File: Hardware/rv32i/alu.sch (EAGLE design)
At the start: 81 parts, among them IC1 SN74HCS86DR, IC10 SN74HCS86DR, IC11 SN74HCS86DR, IC12 SN74HCS86DR, IC13 SN74HCS86DR, IC14 SN74HCS86DR, IC15 SN74HCS86DR, IC16 SN74HCS86DR, IC17 SN74HCS86DR, IC18 SN74HCS86DR, IC19 SN74HCS86DR, IC2 SN74HCS86DR, IC20 SN74HCS86DR, IC21 SN74HCS86DR, IC22 SN74HCS86DR, IC23 SN74HCS86DR, IC24 SN74HCS86DR, IC25 SN74ACT08D, IC26 SN74ACT08D, IC27 SN74ACT08D, IC28 SN74ACT08D, IC29 SN74ACT08D, IC3 SN74HCS86DR, IC30 SN74ACT08D, IC31 SN74ACT08D, IC32 SN74ACT08D, IC33 SN74ACT08D, IC34 SN74ACT08D, IC35 SN74ACT08D, IC36 SN74ACT08D, IC37 SN74ACT08D, IC38 SN74ACT08D, IC39 SN74ACT08D, IC4 SN74HCS86DR, IC40 SN74ACT08D, IC41 SN74HCS32DR, IC42 SN74HCS32DR, IC43 SN74HCS32DR, IC44 SN74HCS32DR, IC45 SN74HCS32DR, IC46 SN74HCS32DR, IC47 SN74HCS32DR, IC48 SN74HCS32DR, IC5 SN74HCS86DR, IC6 SN74HCS86DR, IC7 SN74HCS86DR, IC8 SN74HCS86DR, IC9 SN74HCS86DR

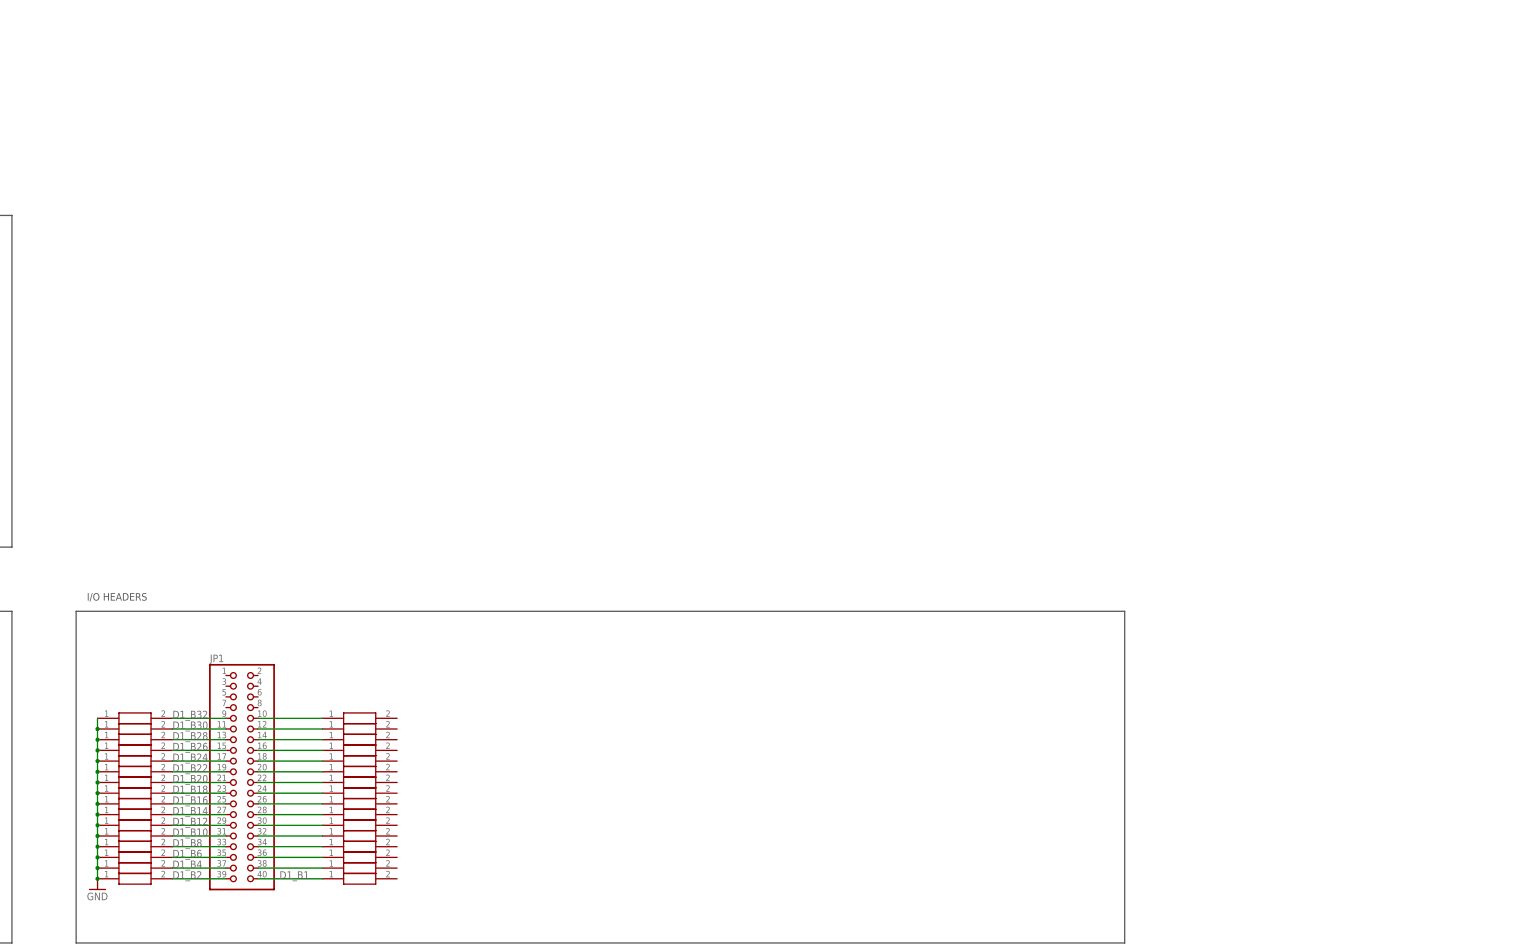
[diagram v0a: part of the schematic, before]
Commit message: ALU Headers & Timing Gates
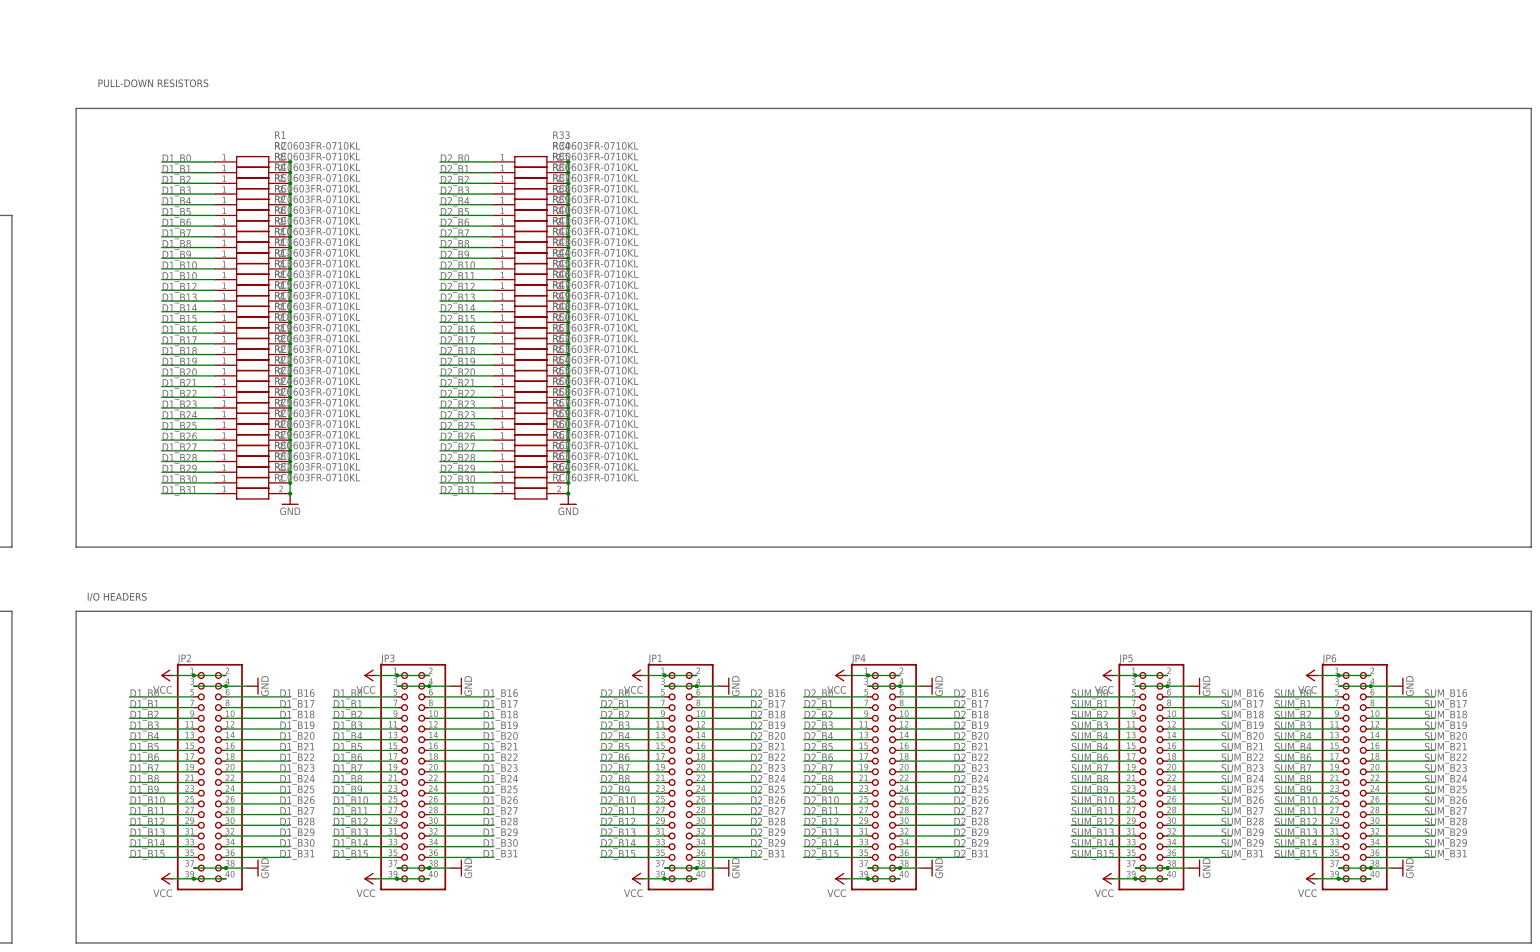
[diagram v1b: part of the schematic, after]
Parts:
- added JP2, JP3, JP4, JP5, JP6: (no value), pinhead:PINHD-2X20
- added R33, R34, R35, R36, R37, R38, R39, R40, R41, R42, R43, R44, R45, R46, R47, R48, R49, R50, R51, R52, R53, R54, R55, R56, R57, R58, R59, R60, R61, R62, R63, R64: RC0603FR-0710KL, RC0603FR-0710KL:RC0603FR-0710KL
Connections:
- removed net N$10: JP1.22, R26.1
- removed net N$11: JP1.24, R25.1
- removed net N$12: JP1.26, R17.1
- removed net N$13: JP1.28, R18.1
- removed net N$14: JP1.30, R19.1
- removed net N$16: JP1.32, R20.1
- removed net N$17: JP1.34, R22.1
- removed net N$18: JP1.36, R21.1
- removed net N$19: JP1.38, R23.1
- removed net N$2: JP1.10, R31.1
- removed net N$4: JP1.12, R32.1
- removed net N$5: JP1.14, R30.1
- removed net N$6: JP1.16, R29.1
- removed net N$7: JP1.18, R28.1
- removed net N$9: JP1.20, R27.1
- new net D1_B0: JP2.5, JP3.5, R1.1
- new net D2_B0: JP1.5, JP4.5, R33.1
- new net SUM_B0: JP5.5, JP6.5
- new net VCC: JP1.1, JP1.2, JP1.39, JP1.40, JP2.1, JP2.2, JP2.39, JP2.40, JP3.1, JP3.2, JP3.39, JP3.40, JP4.1, JP4.2, JP4.39, JP4.40, JP5.1, JP5.2, JP5.39, JP5.40, JP6.1, JP6.2, JP6.39, JP6.40
- net D1_B1: now also JP2.7, JP3.7, R2.1; no longer JP1.40, R24.1
- net D1_B10: now also JP2.25, JP3.25, R11.1, R12.1; no longer JP1.31, R4.2
- net D1_B11: now also JP2.27, JP3.27
- net D1_B12: now also JP2.29, JP3.29, R13.1; no longer JP1.29, R3.2
- net D1_B13: now also JP2.31, JP3.31, R14.1
- net D1_B14: now also JP2.33, JP3.33, R15.1; no longer JP1.27, R2.2
- net D1_B15: now also JP2.35, JP3.35, R17.1
- net D1_B16: now also JP2.6, JP3.6, R16.1; no longer JP1.25, R1.2
- net D1_B17: now also JP2.8, JP3.8, R18.1
- net D1_B18: now also JP2.10, JP3.10, R19.1; no longer JP1.23, R9.2
- net D1_B19: now also JP2.12, JP3.12, R20.1
- net D1_B2: now also JP2.9, JP3.9, R3.1; no longer JP1.39, R8.2
- net D1_B20: now also JP2.14, JP3.14, R21.1; no longer JP1.21, R10.2
- net D1_B21: now also JP2.16, JP3.16, R22.1
- net D1_B22: now also JP2.18, JP3.18, R23.1; no longer JP1.19, R11.2
- net D1_B23: now also JP2.20, JP3.20, R24.1
- net D1_B24: now also JP2.22, JP3.22, R26.1; no longer JP1.17, R12.2
- net D1_B25: now also JP2.24, JP3.24, R25.1
- net D1_B26: now also JP2.26, JP3.26, R27.1; no longer JP1.15, R13.2
- net D1_B27: now also JP2.28, JP3.28, R28.1
- net D1_B28: now also JP2.30, JP3.30, R29.1; no longer JP1.13, R14.2
- net D1_B29: now also JP2.32, JP3.32, R30.1
- net D1_B3: now also JP2.11, JP3.11, R4.1
- net D1_B30: now also JP2.34, JP3.34, R31.1; no longer JP1.11, R16.2
- net D1_B31: now also JP2.36, JP3.36, R32.1
- net D1_B32: no longer JP1.9, R15.2
- net D1_B4: now also JP2.13, JP3.13, R5.1; no longer JP1.37, R7.2
- net D1_B5: now also JP2.15, JP3.15, R6.1
- net D1_B6: now also JP2.17, JP3.17, R7.1; no longer JP1.35, R5.2
- net D1_B7: now also JP2.19, JP3.19, R8.1
- net D1_B8: now also JP2.21, JP3.21, R9.1; no longer JP1.33, R6.2
- net D1_B9: now also JP2.23, JP3.23, R10.1
- net D2_B1: now also JP1.7, JP4.7, R34.1
- net D2_B10: now also JP1.25, JP4.25, R43.1
- net D2_B11: now also JP1.27, JP4.27, R44.1
- net D2_B12: now also JP1.29, JP4.29, R45.1
- net D2_B13: now also JP1.31, JP4.31, R46.1
- net D2_B14: now also JP1.33, JP4.33, R47.1
- net D2_B15: now also JP1.35, JP4.35, R49.1
- net D2_B16: now also JP1.6, JP4.6, R48.1
- net D2_B17: now also JP1.8, JP4.8, R50.1
- net D2_B18: now also JP1.10, JP4.10, R51.1
- net D2_B19: now also JP1.12, JP4.12, R52.1
- net D2_B2: now also JP1.9, JP4.9, R35.1
- net D2_B20: now also JP1.14, JP4.14, R53.1
- net D2_B21: now also JP1.16, JP4.16, R54.1
- net D2_B22: now also JP1.18, JP4.18, R55.1
- net D2_B23: now also JP1.20, JP4.20, R56.1, R58.1
- net D2_B24: now also JP1.22, JP4.22
- net D2_B25: now also JP1.24, JP4.24, R57.1
- net D2_B26: now also JP1.26, JP4.26, R59.1
- net D2_B27: now also JP1.28, JP4.28, R60.1
- net D2_B28: now also JP1.30, JP4.30, R61.1
- net D2_B29: now also JP1.32, JP1.34, JP4.32, JP4.34, R62.1
- net D2_B3: now also JP1.11, JP4.11, R36.1
- net D2_B30: now also R63.1
- net D2_B31: now also JP1.36, JP4.36, R64.1
- net D2_B4: now also JP1.13, JP4.13, R37.1
- net D2_B5: now also JP1.15, JP4.15, R38.1
- net D2_B6: now also JP1.17, JP4.17, R39.1
- net D2_B7: now also JP1.19, JP4.19, R40.1
- net D2_B8: now also JP1.21, JP4.21, R41.1
- net D2_B9: now also JP1.23, JP4.23, R42.1
- net GND: now also JP1.3, JP1.37, JP1.38, JP1.4, JP2.3, JP2.37, JP2.38, JP2.4, JP3.3, JP3.37, JP3.38, JP3.4, JP4.3, JP4.37, JP4.38, JP4.4, JP5.3, JP5.37, JP5.38, JP5.4, JP6.3, JP6.37, JP6.38, JP6.4, R1.2, R10.2, R11.2, R12.2, R13.2, R14.2, R15.2, R16.2, R17.2, R18.2, R19.2, R2.2, R20.2, R21.2, R22.2, R23.2, R24.2, R25.2, R26.2, R27.2, R28.2, R29.2, R3.2, R30.2, R31.2, R32.2, R33.2, R34.2, R35.2, R36.2, R37.2, R38.2, R39.2, R4.2, R40.2, R41.2, R42.2, R43.2, R44.2, R45.2, R46.2, R47.2, R48.2, R49.2, R5.2, R50.2, R51.2, R52.2, R53.2, R54.2, R55.2, R56.2, R57.2, R58.2, R59.2, R6.2, R60.2, R61.2, R62.2, R63.2, R64.2, R7.2, R8.2, R9.2; no longer R1.1, R10.1, R11.1, R12.1, R13.1, R14.1, R15.1, R16.1, R2.1, R3.1, R4.1, R5.1, R6.1, R7.1, R8.1, R9.1
- net SUM_B1: now also JP5.7, JP6.7
- net SUM_B10: now also JP5.25, JP6.25
- net SUM_B11: now also JP5.27, JP6.27
- net SUM_B12: now also JP5.29, JP6.29
- net SUM_B13: now also JP5.31, JP6.31
- net SUM_B14: now also JP5.33, JP6.33
- net SUM_B15: now also JP5.35, JP6.35
- net SUM_B16: now also JP5.6, JP6.6
- net SUM_B17: now also JP5.8, JP6.8
- net SUM_B18: now also JP5.10, JP6.10
- net SUM_B19: now also JP5.12, JP6.12
- net SUM_B2: now also JP5.9, JP6.9
- net SUM_B20: now also JP5.14, JP6.14
- net SUM_B21: now also JP5.16, JP6.16
- net SUM_B22: now also JP5.18, JP6.18
- net SUM_B23: now also JP5.20, JP6.20
- net SUM_B24: now also JP5.22, JP6.22
- net SUM_B25: now also JP5.24, JP6.24
- net SUM_B26: now also JP5.26, JP6.26
- net SUM_B27: now also JP5.28, JP6.28
- net SUM_B28: now also JP5.30, JP6.30
- net SUM_B29: now also JP5.32, JP5.34, JP6.32, JP6.34
- net SUM_B3: now also JP5.11, JP6.11
- net SUM_B31: now also JP5.36, JP6.36
- net SUM_B4: now also JP5.13, JP5.15, JP6.13, JP6.15
- net SUM_B6: now also JP5.17, JP6.17
- net SUM_B7: now also JP5.19, JP6.19
- net SUM_B8: now also JP5.21, JP6.21
- net SUM_B9: now also JP5.23, JP6.23
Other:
- note added: "PULL-DOWN RESISTORS"
- moved on the sheet: JP1
